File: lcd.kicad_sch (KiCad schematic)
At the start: 6 parts, among them J2 LCD 3.2" 240x320 Conn_01x14_P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, Q4 SI2301CDS-T1-GE3

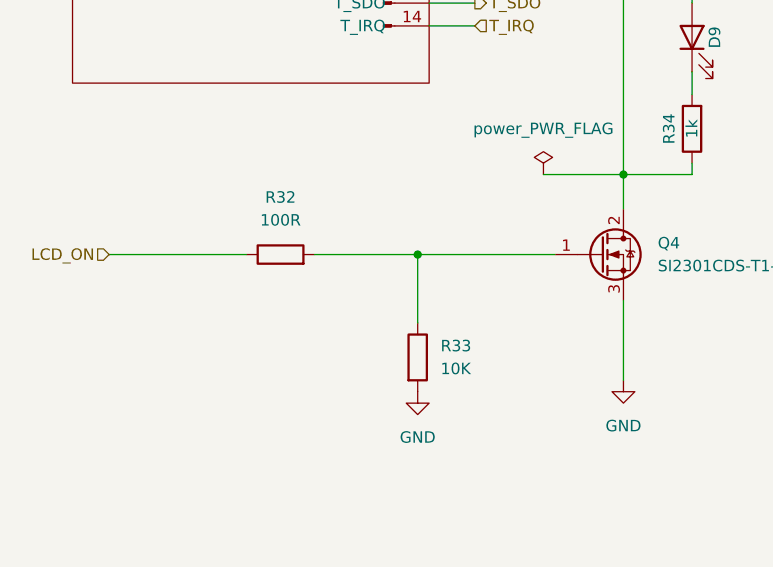
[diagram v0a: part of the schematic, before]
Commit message: remove hellen
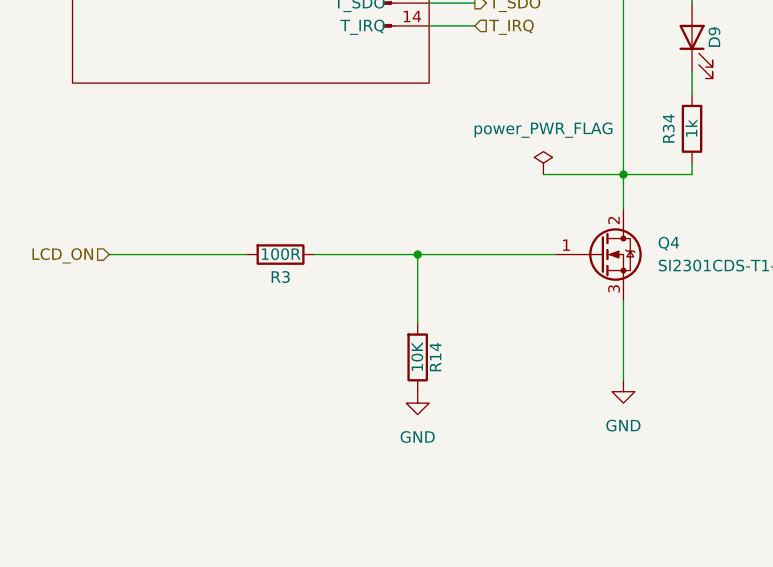
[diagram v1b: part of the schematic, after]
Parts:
- removed R32: 100R, symbol Device:R
- removed R33: 10K, symbol Device:R
- added R14: 10K, Resistor_SMD:R_0603_1608Metric, symbol Device:R
- added R3: 100R, Resistor_SMD:R_0603_1608Metric, symbol Device:R
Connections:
- net GND: now also R14.1
- net LCD_ON: now also R3.2
- net at Q4.1 (G): now also R14.2, R3.1
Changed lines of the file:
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@@
+	)
+	(symbol
+		(lib_id "Device:R")
+		(at 119.38 104.14 270)
+		(unit 1)
+		(exclude_from_sim no)
+		(in_bom yes)
+		(on_board yes)
+		(dnp no)
+		(property "Reference" "R3"
+			(at 119.38 106.68 90)
+			(effects
+				(font
+					(size 1.27 1.27)
+				)
+			)
+		)
+		(property "Value" "100R"
+			(at 119.38 104.14 90)
+			(effects
+				(font
+					(size 1.27 1.27)
+				)
+			)
+		)
+		(property "Footprint" "Resistor_SMD:R_0603_1608Metric"
+			(at 119.38 102.362 90)
+			(effects
+				(font
+					(size 1.27 1.27)
+				)
+				(hide yes)
+			)
+		)
+		(property "Datasheet" "~"
+			(at 119.38 104.14 0)
+			(effects
+				(font
+					(size 1.27 1.27)
+				)
+				(hide yes)
+			)
+		)
+		(property "Description" "Resistor"
+			(at 119.38 104.14 0)
+			(effects
+				(font
+					(size 1.27 1.27)
+				)
+				(hide yes)
+			)
+		)
+		(property "LCSC" "C21190"
+			(at 119.38 104.14 0)
+			(effects
+				(font
+					(size 1.27 1.27)
+				)
+				(hide yes)
+			)
+		)
+		(property "Manufacturer" "StackPole"
+			(at 119.38 104.14 0)
+			(effects
+				(font
+					(size 1.27 1.27)
+				)
+				(hide yes)
+			)
+		)
+		(property "Part #" "RMCF0603JJ1K00"
+			(at 119.38 104.14 0)
+			(effects
+				(font
+					(size 1.27 1.27)
+				)
+				(hide yes)
+			)
+		)
+		(property "VEND" "DIGI"
+			(at 119.38 104.14 0)
+			(effects
+				(font
+					(size 1.27 1.27)
+				)
+				(hide yes)
+			)
+		)
+		(property "VEND#" "RMCF0603JJ1K00CT-ND"
+			(at 119.38 104.14 0)
+			(effects
+				(font
+					(size 1.27 1.27)
+				)
+				(hide yes)
+			)
+		)
+		(pin "1"
+		)
+		(pin "2"
+		)
+		(instances
+			(project "l8-kicad"
+				(path "/8d063f79-9282-4820-bcf4-1ff3c006cf08/98bf8f66-79b9-41fc-9cd7-550fbae3319a"
+					(reference "R3")
+					(unit 1)
+				)
+			)
+		)
 	)
 	(symbol
@@
 	(symbol
 		(lib_id "Device:R")
-		(at 119.38 104.14 90)
+		(at 134.62 115.57 0)
+		(mirror x)
 		(unit 1)
 		(exclude_from_sim no)
@@
 		(on_board yes)
 		(dnp no)
-		(fields_autoplaced yes)
-		(property "Reference" "R32"
-			(at 119.38 97.79 90)
-			(effects
-				(font
-					(size 1.27 1.27)
-				)
-			)
-		)
-		(property "Value" "100R"
-			(at 119.38 100.33 90)
-			(effects
-				(font
-					(size 1.27 1.27)
-				)
-			)
-		)
-		(property "Footprint" ""
-			(at 119.38 105.918 90)
-			(effects
-				(font
-					(size 1.27 1.27)
+		(property "Reference" "R14"
+			(at 136.652 115.57 90)
+			(effects
+				(font
+					(size 1.27 1.27)
+				)
+			)
+		)
+		(property "Value" "10K"
+			(at 134.62 115.57 90)
+			(effects
+				(font
+					(size 1.27 1.27)
+				)
+			)
+		)
+		(property "Footprint" "Resistor_SMD:R_0603_1608Metric"
+			(at 193.802 173.99 90)
+			(effects
+				(font
+					(size 1.524 1.524)
 				)
 				(hide yes)
@@
 		)
 		(property "Datasheet" "~"
-			(at 119.38 104.14 0)
-			(effects
-				(font
-					(size 1.27 1.27)
+			(at 283.21 174.625 0)
+			(effects
+				(font
+					(size 1.524 1.524)
 				)
 				(hide yes)
@@
 		)
 		(property "Description" "Resistor"
-			(at 119.38 104.14 0)
+			(at 134.62 115.57 0)
+			(effects
+				(font
+					(size 1.27 1.27)
+				)
+				(hide yes)
+			)
+		)
+		(property "Part #" "RMCF0603JT10K0"
+			(at 16.51 8.89 0)
+			(effects
+				(font
+					(size 1.27 1.27)
+				)
+				(hide yes)
+			)
+		)
+		(property "VEND" "DIGI"
+			(at 16.51 8.89 0)
+			(effects
+				(font
+					(size 1.27 1.27)
+				)
+				(hide yes)
+			)
+		)
+		(property "VEND#" "RMCF0603JT10K0CT-ND"
+			(at 16.51 8.89 0)
+			(effects
+				(font
+					(size 1.27 1.27)
+				)
+				(hide yes)
+			)
+		)
+		(property "Manufacturer" "StackPole"
+			(at 16.51 8.89 0)
+			(effects
+				(font
+					(size 1.27 1.27)
+				)
+				(hide yes)
+			)
+		)
+		(property "LCSC" "C25804"
+			(at 134.62 115.57 0)
 			(effects
 				(font
@@
 			(project "l8-kicad"
 				(path "/8d063f79-9282-4820-bcf4-1ff3c006cf08/98bf8f66-79b9-41fc-9cd7-550fbae3319a"
-					(reference "R32")
+					(reference "R14")
 					(unit 1)
 				)
@@
 					(unit 1)
 				)
-			)
-		)
-	)
-	(symbol
-		(lib_id "Device:R")
-		(at 134.62 115.57 0)
-		(unit 1)
-		(exclude_from_sim no)
-		(in_bom yes)
-		(on_board yes)
-		(dnp no)
-		(fields_autoplaced yes)
-		(property "Reference" "R33"
-			(at 137.16 114.2999 0)
-			(effects
-				(font
-					(size 1.27 1.27)
-				)
-				(justify left)
-			)
-		)
-		(property "Value" "10K"
-			(at 137.16 116.8399 0)
-			(effects
-				(font
-					(size 1.27 1.27)
-				)
-				(justify left)
-			)
-		)
-		(property "Footprint" ""
-			(at 132.842 115.57 90)
-			(effects
-				(font
-					(size 1.27 1.27)
-				)
-				(hide yes)
-			)
-		)
-		(property "Datasheet" "~"
-			(at 134.62 115.57 0)
-			(effects
-				(font
-					(size 1.27 1.27)
-				)
-				(hide yes)
-			)
-		)
-		(property "Description" "Resistor"
-			(at 134.62 115.57 0)
-			(effects
-				(font
-					(size 1.27 1.27)
-				)
-				(hide yes)
-			)
-		)
-		(pin "1"
-		)
-		(pin "2"
-		)
-		(instances
-			(project "l8-kicad"
-				(path "/8d063f79-9282-4820-bcf4-1ff3c006cf08/98bf8f66-79b9-41fc-9cd7-550fbae3319a"
-					(reference "R33")
-					(unit 1)
-				)
